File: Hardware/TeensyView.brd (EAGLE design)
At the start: 35.6 x 17.8 mm, 23 parts, among them J1 DNP, J2 DNP

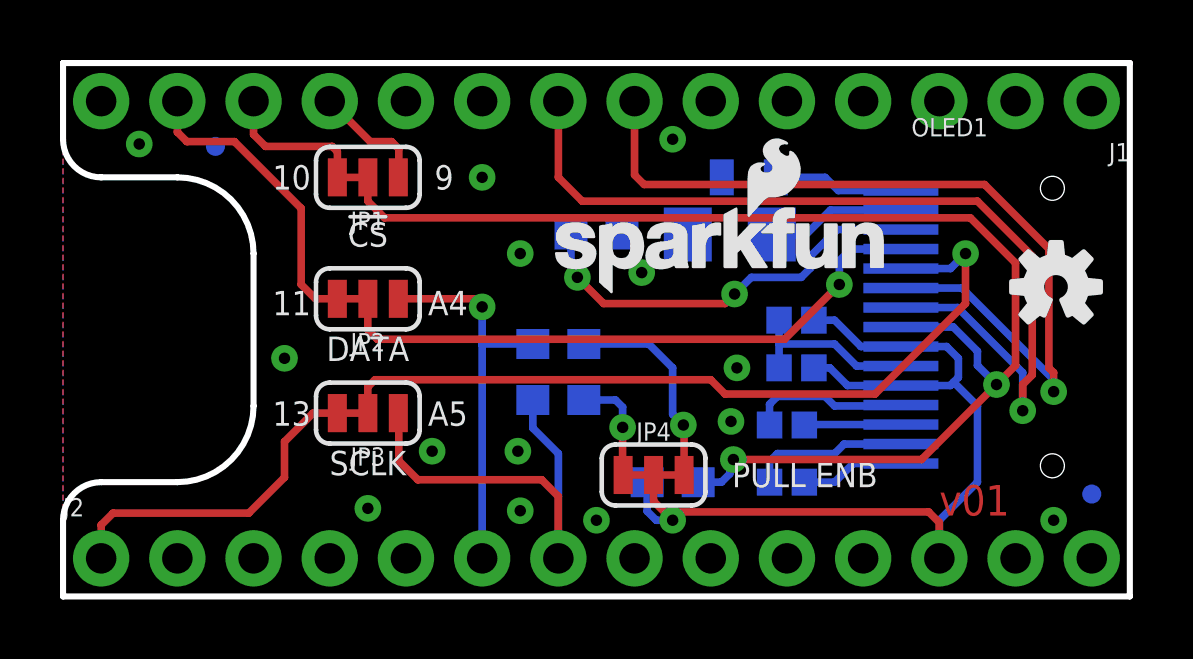
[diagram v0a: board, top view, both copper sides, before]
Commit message: Going for proto 2
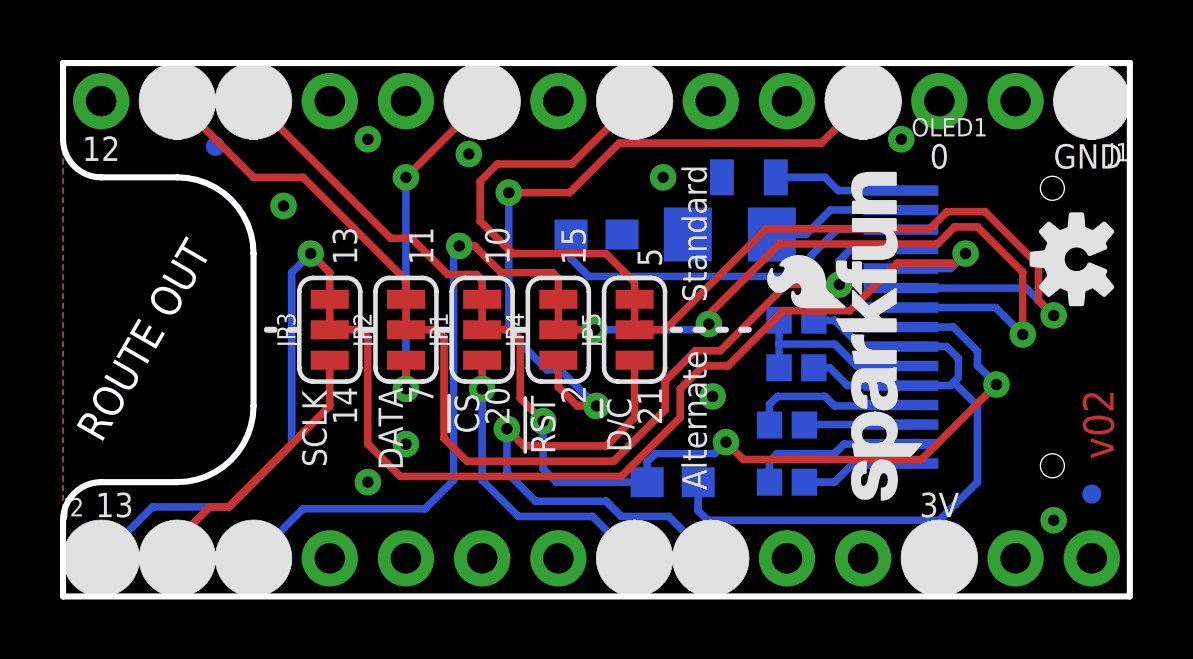
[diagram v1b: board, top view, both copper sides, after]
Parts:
- removed R2, R3: 4.7k, SparkFun-Resistors:0603
- added JP5: JUMPER-SMT_3_1-NC_TRACE_SILK, SparkFun-Jumpers:SMT-JUMPER_3_1-NC_TRACE_SILK
- JP4: value JUMPER-SMT_3_2-NC_TRACE_SILK -> JUMPER-SMT_3_1-NC_TRACE_SILK; device SparkFun-Jumpers:SMT-JUMPER_3_2-NC_TRACE_SILK -> SparkFun-Jumpers:SMT-JUMPER_3_1-NC_TRACE_SILK
- moved LOGO3 14.6 mm to (28.7, 2.79), turned to 90 degrees
- moved JP1 6.35 mm to (14.0, 8.89), turned to 90 degrees
- moved JP4 5.79 mm to (16.5, 8.89), turned to 90 degrees
- moved JP3 3.05 mm to (8.89, 8.89), turned to 90 degrees
- moved JP2 1.64 mm to (11.4, 8.89), turned to 90 degrees
- moved LOGO2 1.15 mm to (33.8, 11.2), turned to 90 degrees
- turned R4 to 180 degrees
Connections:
- removed net A4PU: JP4.3, R2.2
- removed net A5PU: JP4.1, R3.2
- new net N$14: J2.3, JP4.3
- new net N$15: J1.4, JP4.1
- new net N$16: J1.7, JP5.3
- new net N$17: J2.9, JP5.1
- net !RESET: now also JP4.2; no longer J1.8
- net D/!C: now also JP5.2; no longer J1.7
- net N$11: now also J2.2; no longer J2.7, R3.1
- net N$13: now also J1.9; no longer J2.6, R2.1
- net N$2: now also J2.8; no longer J1.11
- net VCC: no longer JP4.2
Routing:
- net N$15: track 0.00 -> 24.1 mm, vias 0 -> 2
- net N$14: track 0.00 -> 20.1 mm, vias 0 -> 1
- net N$17: track 0.00 -> 16.2 mm, vias 0 -> 1
- net !CS: track 43.3 -> 27.8 mm, vias 2 -> 3
- net N$16: track 0.00 -> 14.1 mm
- net A4PU: track 7.02 -> 0.00 mm, vias 1 -> 0
- net !RESET: track 30.9 -> 24.2 mm, vias 1 -> 3
- net N$2: track 3.92 -> 10.2 mm, vias 0 -> 1
- net N$11: track 15.1 -> 9.08 mm
- net N$1: track 5.00 -> 10.7 mm
- net D/!C: track 28.9 -> 23.2 mm
- net N$10: track 11.2 -> 16.3 mm, vias 0 -> 1
- net VCC: track 32.0 -> 27.0 mm, vias 1 -> 0
- net SCLK: track 26.4 -> 31.3 mm
- net A5PU: track 3.66 -> 0.00 mm, vias 1 -> 0
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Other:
- board text added: "!RST"
- board text added: "0"
- board text added: "12"
- board text added: "14"
- board text added: "15"
- board text added: "2"
- board text added: "20"
- board text added: "21"
- board text added: "3V"
- board text added: "5"
- board text added: "7"
- board text added: "Alternate"
- board text added: "D/!C"
- board text added: "G"
- board text added: "GND"
- board text added: "ROUTE OUT"
- board text added: "Standard"
- board text added: "v02"
- board text removed: "9"
- board text removed: "A4"
- board text removed: "A5"
- board text removed: "PULL ENB"
- board text removed: "v01"
